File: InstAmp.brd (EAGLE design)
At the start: 77.5 x 54.3 mm, 37 parts, among them IC1 AD8221ARZ, IC2 TLC2254ID

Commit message: Rename lbr
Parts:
- IC1: device nanoeeg:AD8221ARZ -> femtoexg:AD8221ARZ
- IC2: device nanoeeg:TLC2254ID -> femtoexg:TLC2254ID
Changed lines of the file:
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@@
 <element name="R5" library="rcl" package="R0805" value="2k2" x="17.78" y="17.78" rot="MR180"/>
 <element name="R6" library="rcl" package="R0805" value="2k2" x="17.78" y="5.08" rot="MR180"/>
-<element name="IC1" library="nanoeeg" package="AD8221ARZ" value="AD8221ARZ" x="22.86" y="11.43" rot="MR90"/>
+<element name="IC1" library="femtoexg" package="AD8221ARZ" value="AD8221ARZ" x="22.86" y="11.43" rot="MR90"/>
 <element name="R7" library="rcl" package="R0805" value="2k" x="17.78" y="11.43" rot="MR270"/>
 <element name="C4" library="rcl" package="C0805" value="0.1" x="73.66" y="24.13"/>
 <element name="C5" library="rcl" package="C0805" value="0.1" x="60.96" y="44.45"/>
-<element name="IC2" library="nanoeeg" package="TLC2254ID" value="TLC2254ID" x="33.02" y="25.4" rot="R90"/>
+<element name="IC2" library="femtoexg" package="TLC2254ID" value="TLC2254ID" x="33.02" y="25.4" rot="R90"/>
 <element name="R8" library="rcl" package="R0805" value="100k" x="24.13" y="33.02"/>
 <element name="R9" library="rcl" package="R0805" value="100k" x="30.48" y="39.37"/>

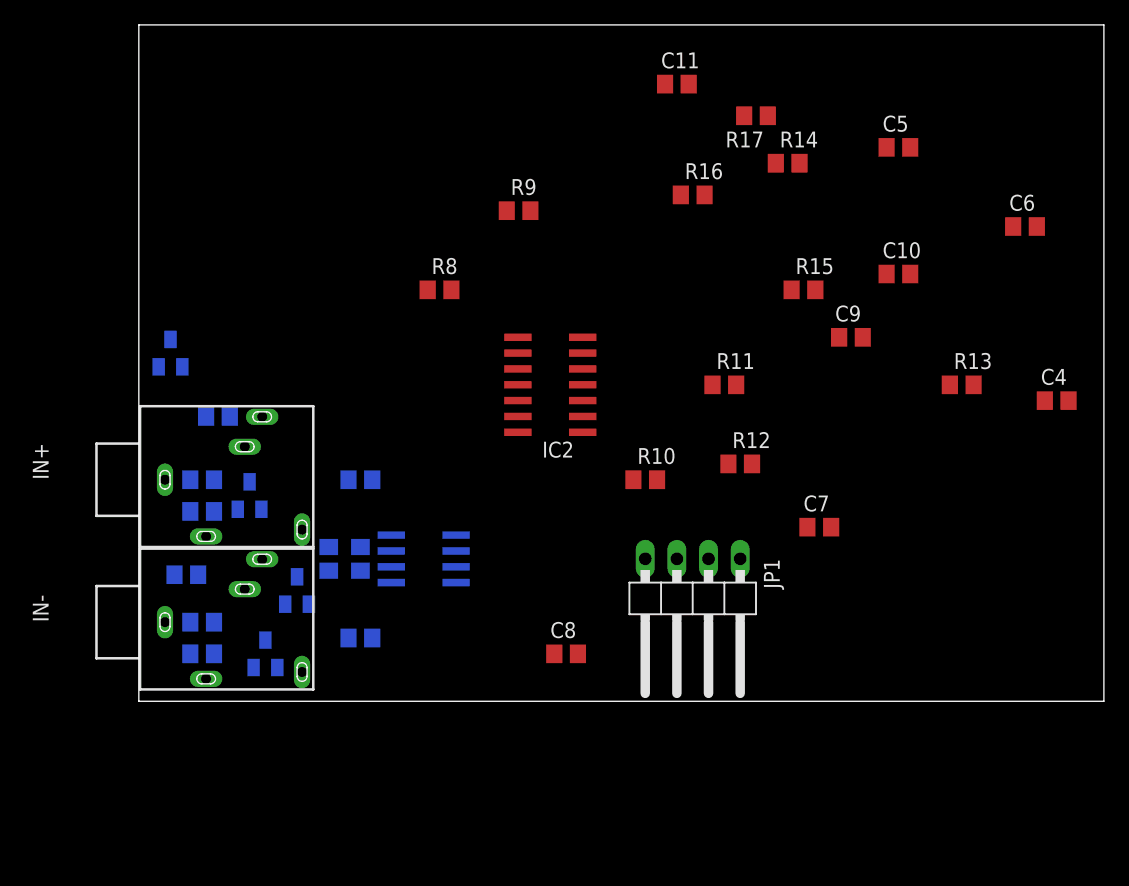
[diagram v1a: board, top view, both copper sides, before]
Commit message: Dimensions
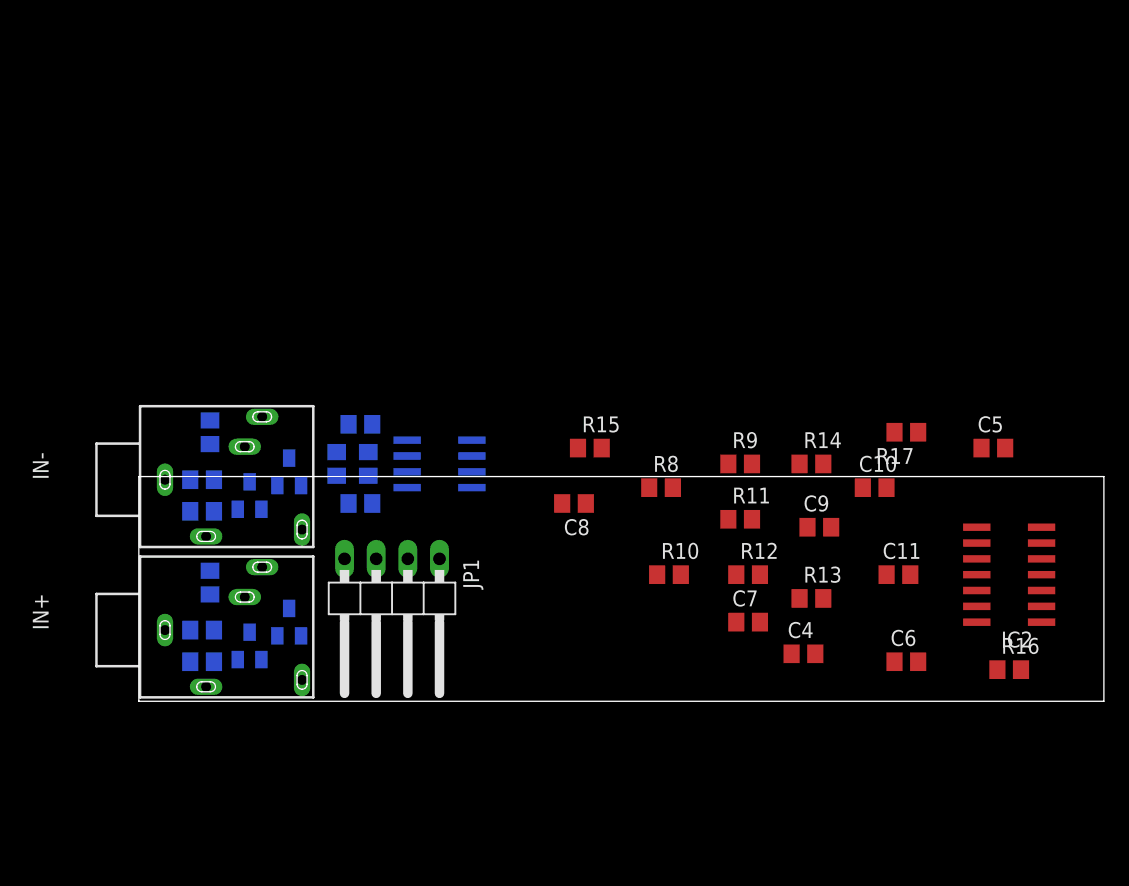
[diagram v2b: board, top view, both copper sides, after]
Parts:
- JP1: value (none) -> OUT
- moved R16 45.8 mm to (69.8, 2.54)
- moved C11 43.2 mm to (61.0, 10.2)
- moved IC2 39.9 mm to (69.8, 10.2)
- moved C6 36.2 mm to (61.6, 3.17)
- moved C4 28.7 mm to (53.3, 3.81)
- moved R17 28.1 mm to (61.6, 21.6)
- moved R9 27.0 mm to (48.3, 19.1)
- moved C5 25.3 mm to (68.6, 20.3)
- moved R14 24.2 mm to (54.0, 19.1)
- moved JP1 24.1 mm to (20.3, 7.62)
- moved R8 23.8 mm to (41.9, 17.1)
- moved D2 23.6 mm to (12.1, 6.35)
- moved R15 21.3 mm to (36.2, 20.3)
- moved R13 21.0 mm to (54.0, 8.26)
- moved C10 17.3 mm to (59.1, 17.1)
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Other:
- board size 77.5 x 54.3 mm -> 77.5 x 18 mm

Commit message: Routing
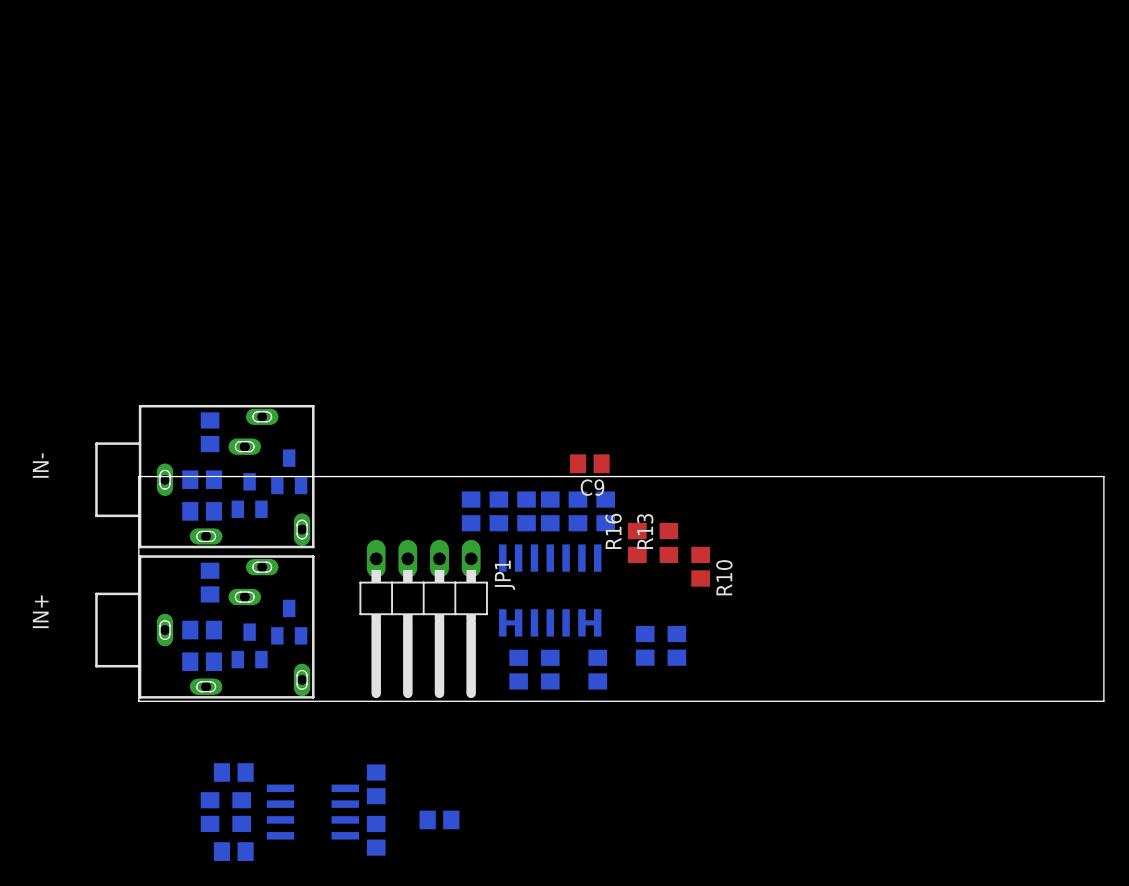
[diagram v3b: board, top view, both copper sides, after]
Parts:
- C4, C5, C6, C7: value 0.1 -> 0.1uF
- moved C5 58.5 mm to (19.1, -10.8), flipped to the bottom, turned to 270 degrees
- moved C11 41.8 mm to (24.1, -9.53), flipped to the bottom
- moved IC2 36.9 mm to (33.0, 8.89), flipped to the bottom, turned to 180 degrees
- moved C4 35.9 mm to (19.1, -6.67), flipped to the bottom, turned to 270 degrees
- moved R16 31.5 mm to (40.0, 12.7), turned to 90 degrees
- moved C6 31.0 mm to (33.0, 15.2), flipped to the bottom, turned to 90 degrees
- moved C1 29.7 mm to (5.71, -8.89)
- moved IC1 29.7 mm to (14.0, -8.89)
- moved R6 29.7 mm to (7.62, -5.71)
- moved R7 29.7 mm to (8.26, -8.89)
- moved R5 29.7 mm to (7.62, -12.1)
- moved R17 25.0 mm to (37.5, 15.2), flipped to the bottom, turned to 270 degrees
- moved R9 24.3 mm to (30.5, 2.54), flipped to the bottom, turned to 270 degrees
- moved C10 22.4 mm to (40.6, 4.45), flipped to the bottom, turned to 270 degrees
- moved R11 21.6 mm to (26.7, 15.2), flipped to the bottom, turned to 270 degrees
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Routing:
- net N$10: track 0.00 -> 1.27 mm
- net N$9: track 0.00 -> 1.27 mm
